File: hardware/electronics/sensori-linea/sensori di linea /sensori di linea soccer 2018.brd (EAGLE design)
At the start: 88.1 x 42 mm, 27 parts, among them T1 BP103, T2 BP103, T3 BP103, T4 BP103

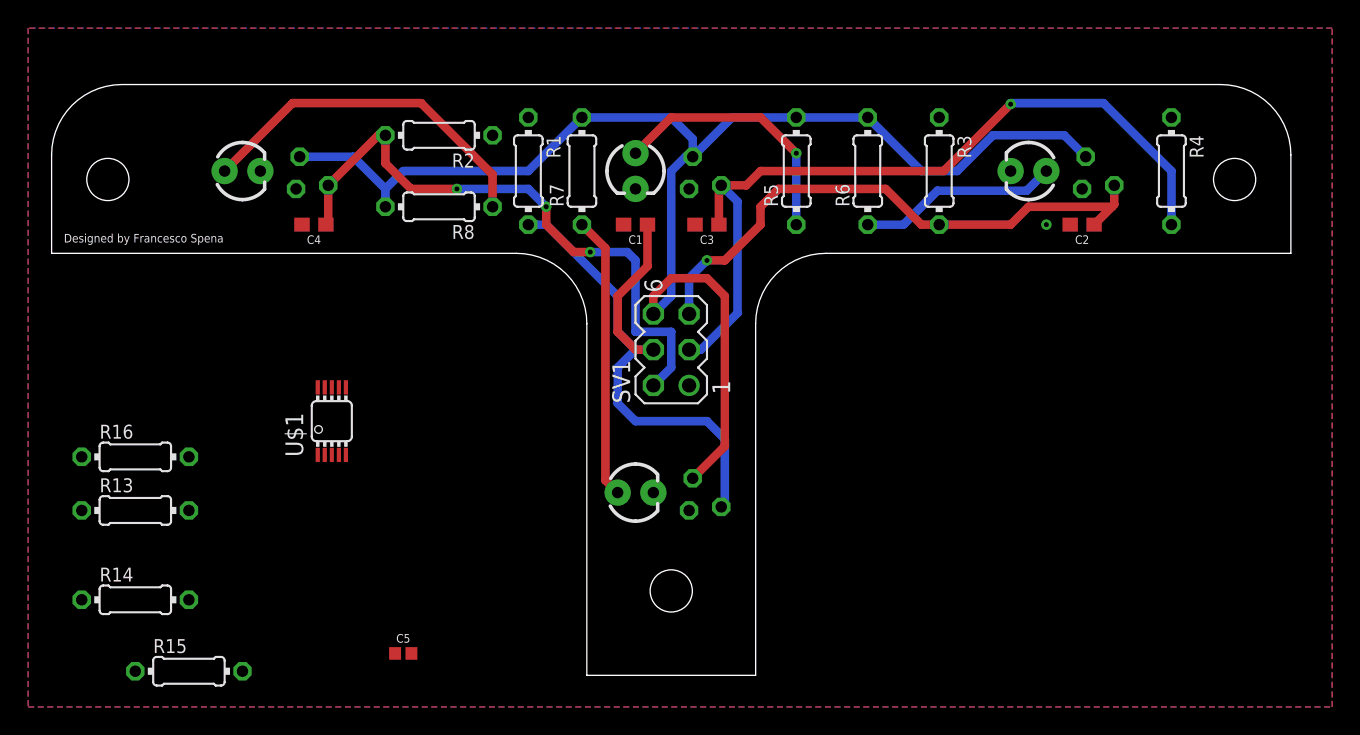
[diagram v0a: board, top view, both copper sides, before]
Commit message: modifiche
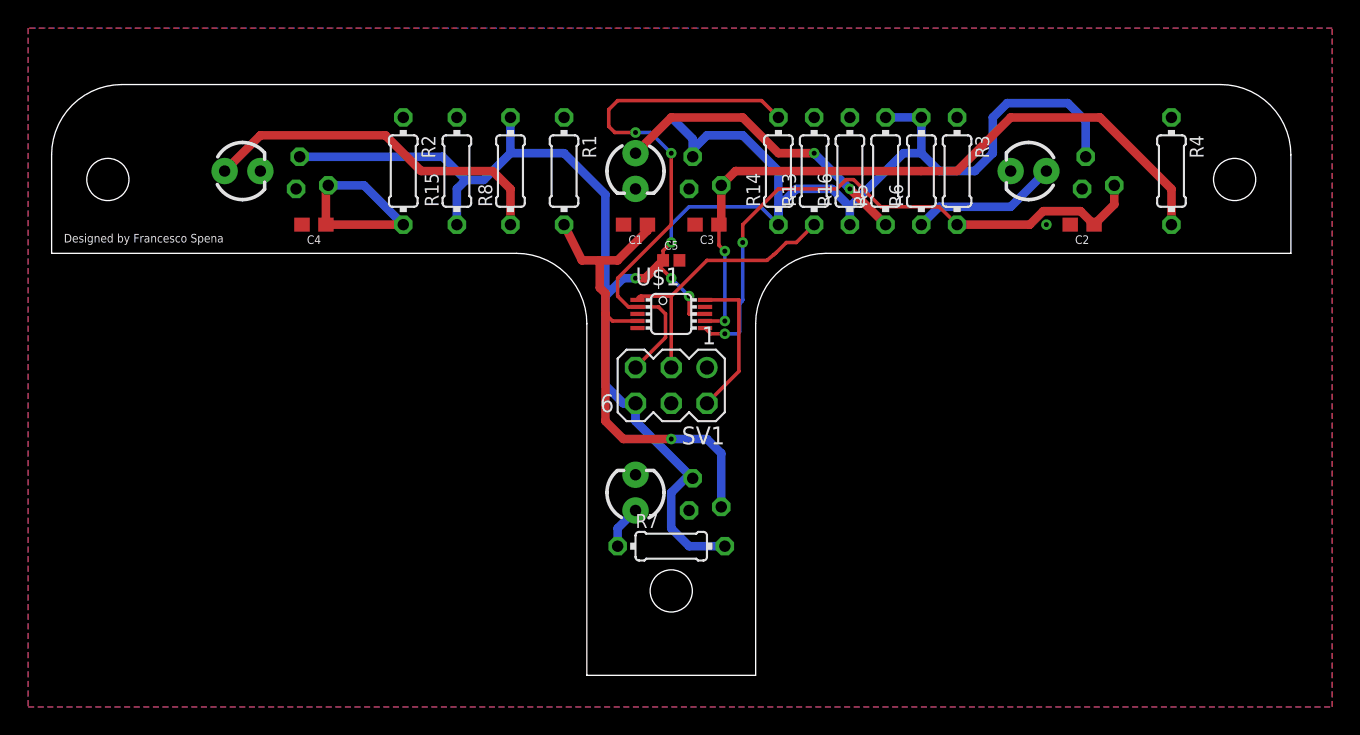
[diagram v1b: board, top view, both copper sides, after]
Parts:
- moved R14 54.9 mm to (7.62, 69.8), turned to 90 degrees
- moved R16 54.7 mm to (12.7, 69.8), turned to 90 degrees
- moved R13 54.0 mm to (10.2, 69.8), turned to 90 degrees
- moved R15 40.3 mm to (-15.2, 69.8), turned to 90 degrees
- moved C5 33.8 mm to (0.00, 63.5)
- moved R7 27.4 mm to (0.00, 43.2), turned to 0 degrees
- moved U$1 25.3 mm to (0.00, 59.7), turned to 270 degrees
- moved R5 6.35 mm to (15.2, 69.8)
- moved R8 5.68 mm to (-11.4, 69.8), turned to 90 degrees
- moved R6 3.81 mm to (17.8, 69.8)
- moved R2 3.59 mm to (-19.1, 69.8), turned to 270 degrees
- moved R1 2.54 mm to (-7.62, 69.8)
- moved SV1 2.54 mm to (0.00, 54.6), turned to 180 degrees
- moved R3 1.27 mm to (20.3, 69.8)
- turned D7 to 90 degrees
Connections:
- removed net N$1: R13.1, U$1.1
- removed net N$6: R16.2, U$1.9
- removed net N$7: R14.2, U$1.2
- removed net N$8: R15.2, U$1.10
- new net ADDR: R13.1, SV1.3, U$1.1
- new net ALERT: R14.2, SV1.5, U$1.2
- new net SCL: R15.2, SV1.2, U$1.10
- new net SDA: R16.2, SV1.4, U$1.9
- net OUT1: no longer SV1.4
- net OUT2: no longer SV1.2
- net OUT3: no longer SV1.5
- net OUT4: no longer SV1.3
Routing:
- net ALERT: track 0.00 -> 39.6 mm, vias 0 -> 2
- net VCC: track 100.5 -> 138.9 mm, vias 0 -> 4
- net OUT2: track 43.7 -> 14.9 mm, vias 3 -> 0
- net ADDR: track 0.00 -> 19.8 mm
- net N$4: track 20.1 -> 3.07 mm
- net SCL: track 0.00 -> 10.7 mm
- net OUT1: track 43.6 -> 35.9 mm, vias 0 -> 1
- net OUT4: track 57.2 -> 50.0 mm, vias 1 -> 2
- net N$3: track 14.3 -> 10.5 mm
- net N$2: track 18.6 -> 22.0 mm, vias 1 -> 2
- net OUT3: track 40.9 -> 42.5 mm, vias 1 -> 2
